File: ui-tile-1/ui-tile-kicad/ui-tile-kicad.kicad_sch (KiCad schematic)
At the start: 0 parts

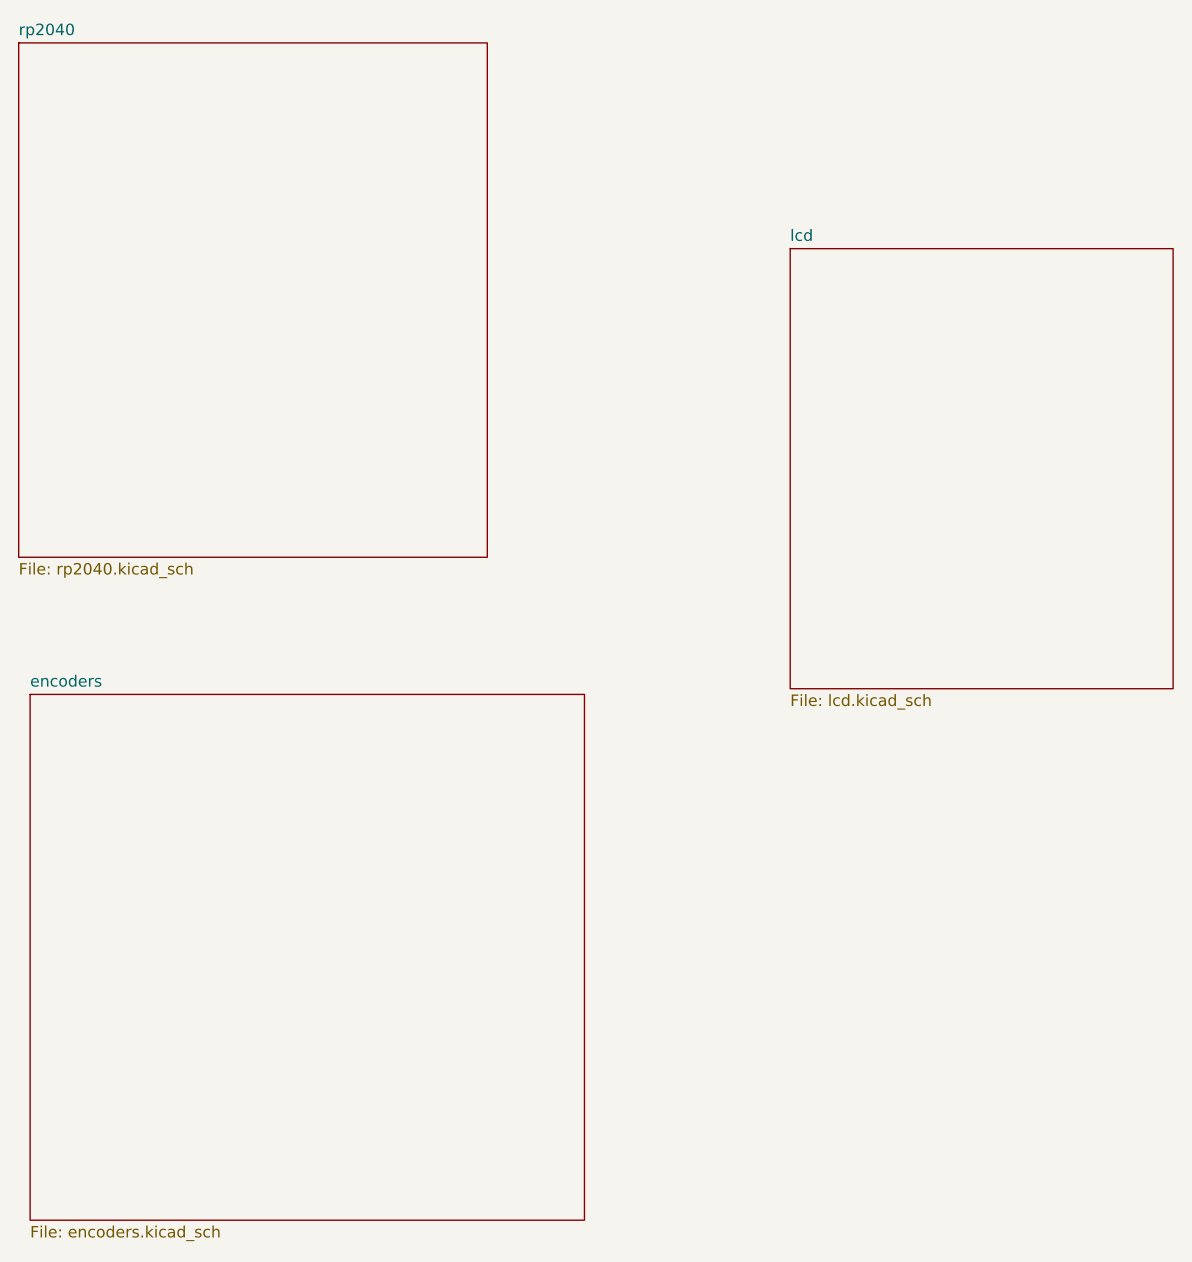
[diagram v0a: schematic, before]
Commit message: finished schematic electricals
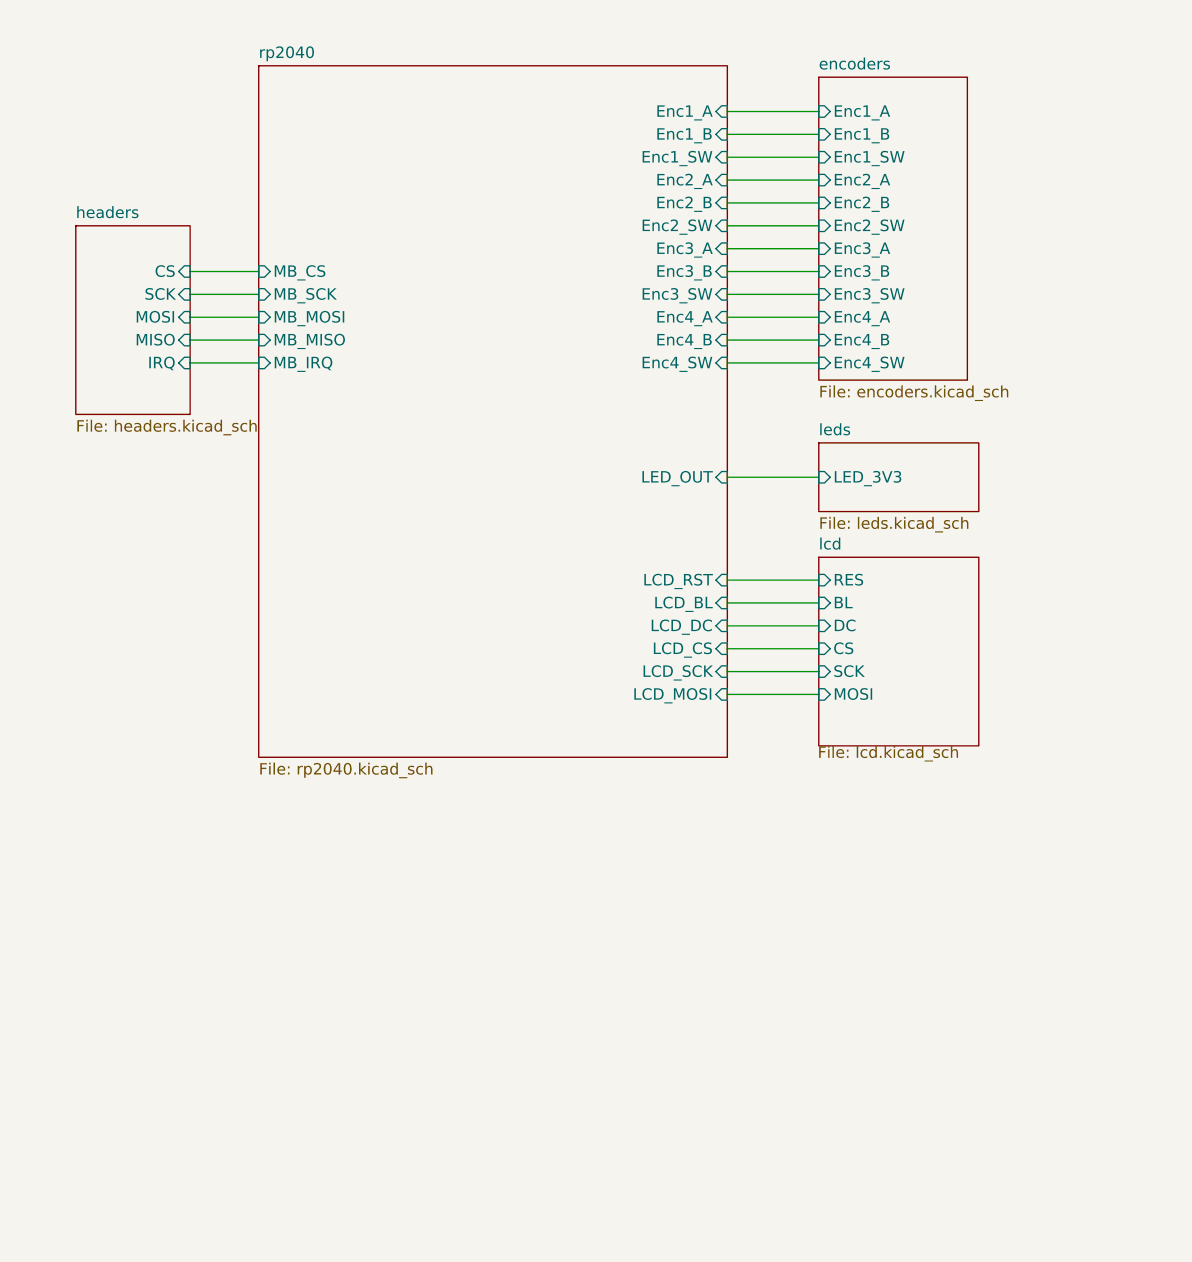
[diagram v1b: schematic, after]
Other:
- added sheet headers (headers.kicad_sch)
- added sheet leds (leds.kicad_sch)
- sheet encoders ports: added Enc1_A, Enc1_B, Enc1_SW, Enc2_A, Enc2_B, Enc2_SW, Enc3_A, Enc3_B, Enc3_SW, Enc4_A, Enc4_B, Enc4_SW; removed none
- sheet lcd ports: added BL, CS, DC, MOSI, RES, SCK; removed none
- sheet rp2040 ports: added Enc1_A, Enc1_B, Enc1_SW, Enc2_A, Enc2_B, Enc2_SW, Enc3_A, Enc3_B, Enc3_SW, Enc4_A, Enc4_B, Enc4_SW, LCD_BL, LCD_CS, LCD_DC, LCD_MOSI, LCD_RST, LCD_SCK, LED_OUT, MB_CS, MB_IRQ, MB_MISO, MB_MOSI, MB_SCK; removed none
